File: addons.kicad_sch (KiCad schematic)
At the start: 4 parts, among them J8 Conn_01x04_MountingPin, J9 Conn_02x03_Odd_Even

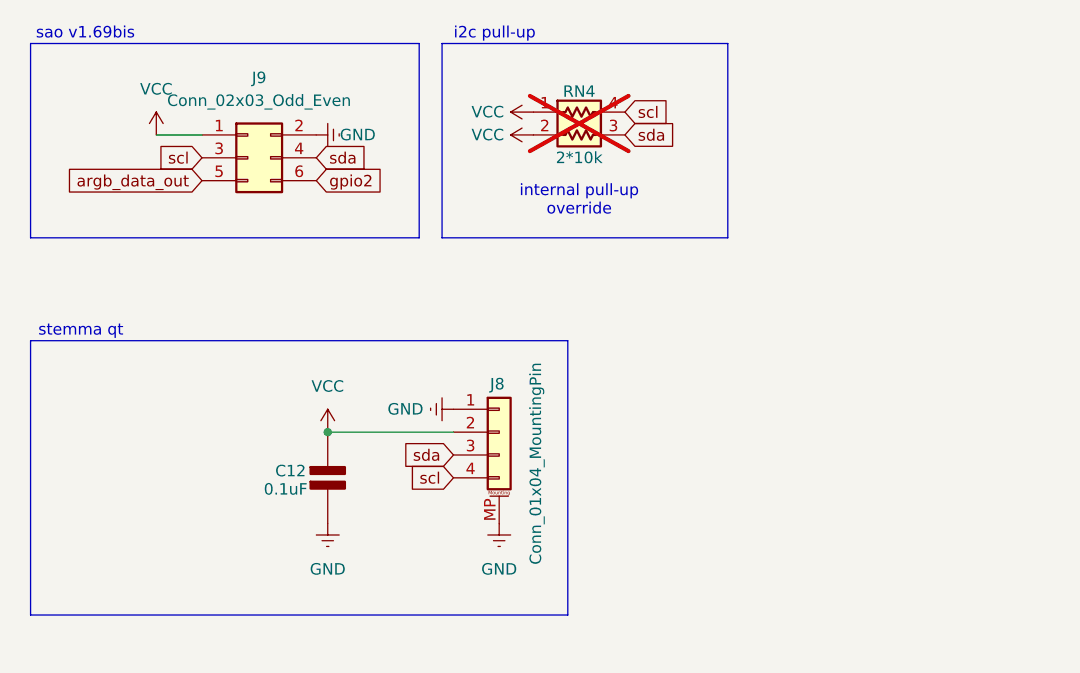
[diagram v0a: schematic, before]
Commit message: progress
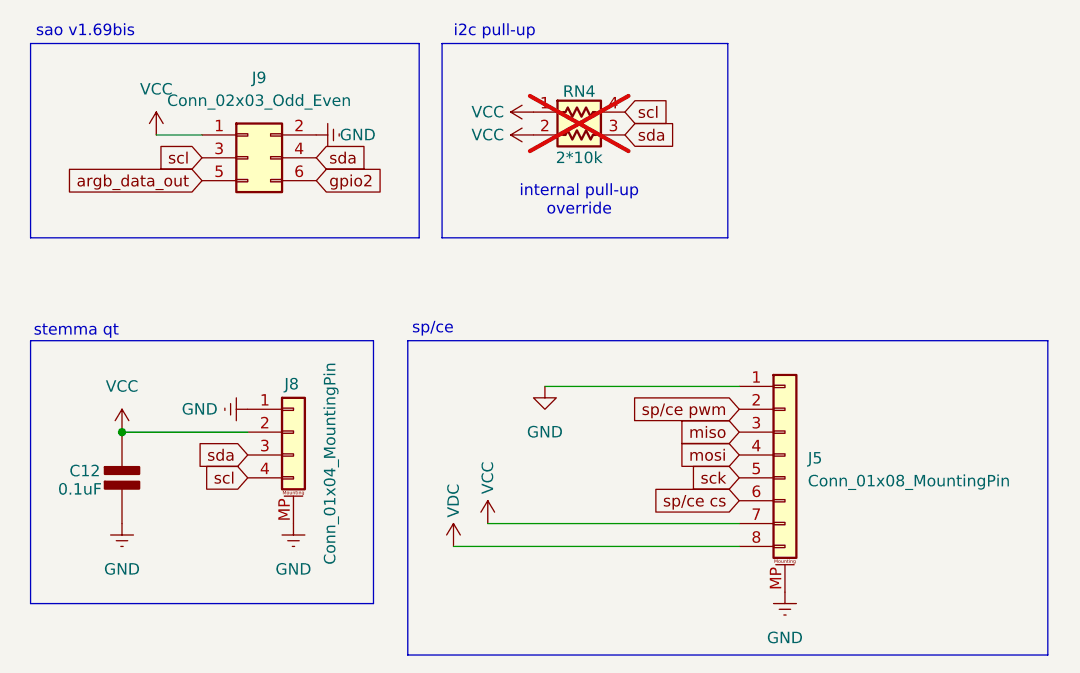
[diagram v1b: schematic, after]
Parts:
- added J5: Conn_01x08_MountingPin, Connector_JST:JST_SH_SM08B-SRSS-TB_1x08-1MP_P1.00mm_Horizontal, symbol Connector_Generic_MountingPin:Conn_01x08_MountingPin
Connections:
- net GND: now also J5.1 (Pin_1), J5.MP (MountPin)
- net VCC: now also J5.7 (Pin_7)
- new net VDC: J5.8 (Pin_8)
- new net miso: J5.3 (Pin_3)
- new net mosi: J5.4 (Pin_4)
- new net sck: J5.5 (Pin_5)
- new net sp/ce cs: J5.6 (Pin_6)
- new net sp/ce pwm: J5.2 (Pin_2)
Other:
- note added: "sp/ce"
- moved on the sheet: C12, J8
